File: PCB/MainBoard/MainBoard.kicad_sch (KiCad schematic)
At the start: 15 parts, among them J1 Conn_01x04_12864, J2 Conn_01x03_Female, J3 Conn_01x03_Female, J4 Conn_01x04_12864, J5 Conn_01x04_12864, J6 Conn_02x20_Odd_Even, SW1 RotaryEncoder_Switch, U2 Pico

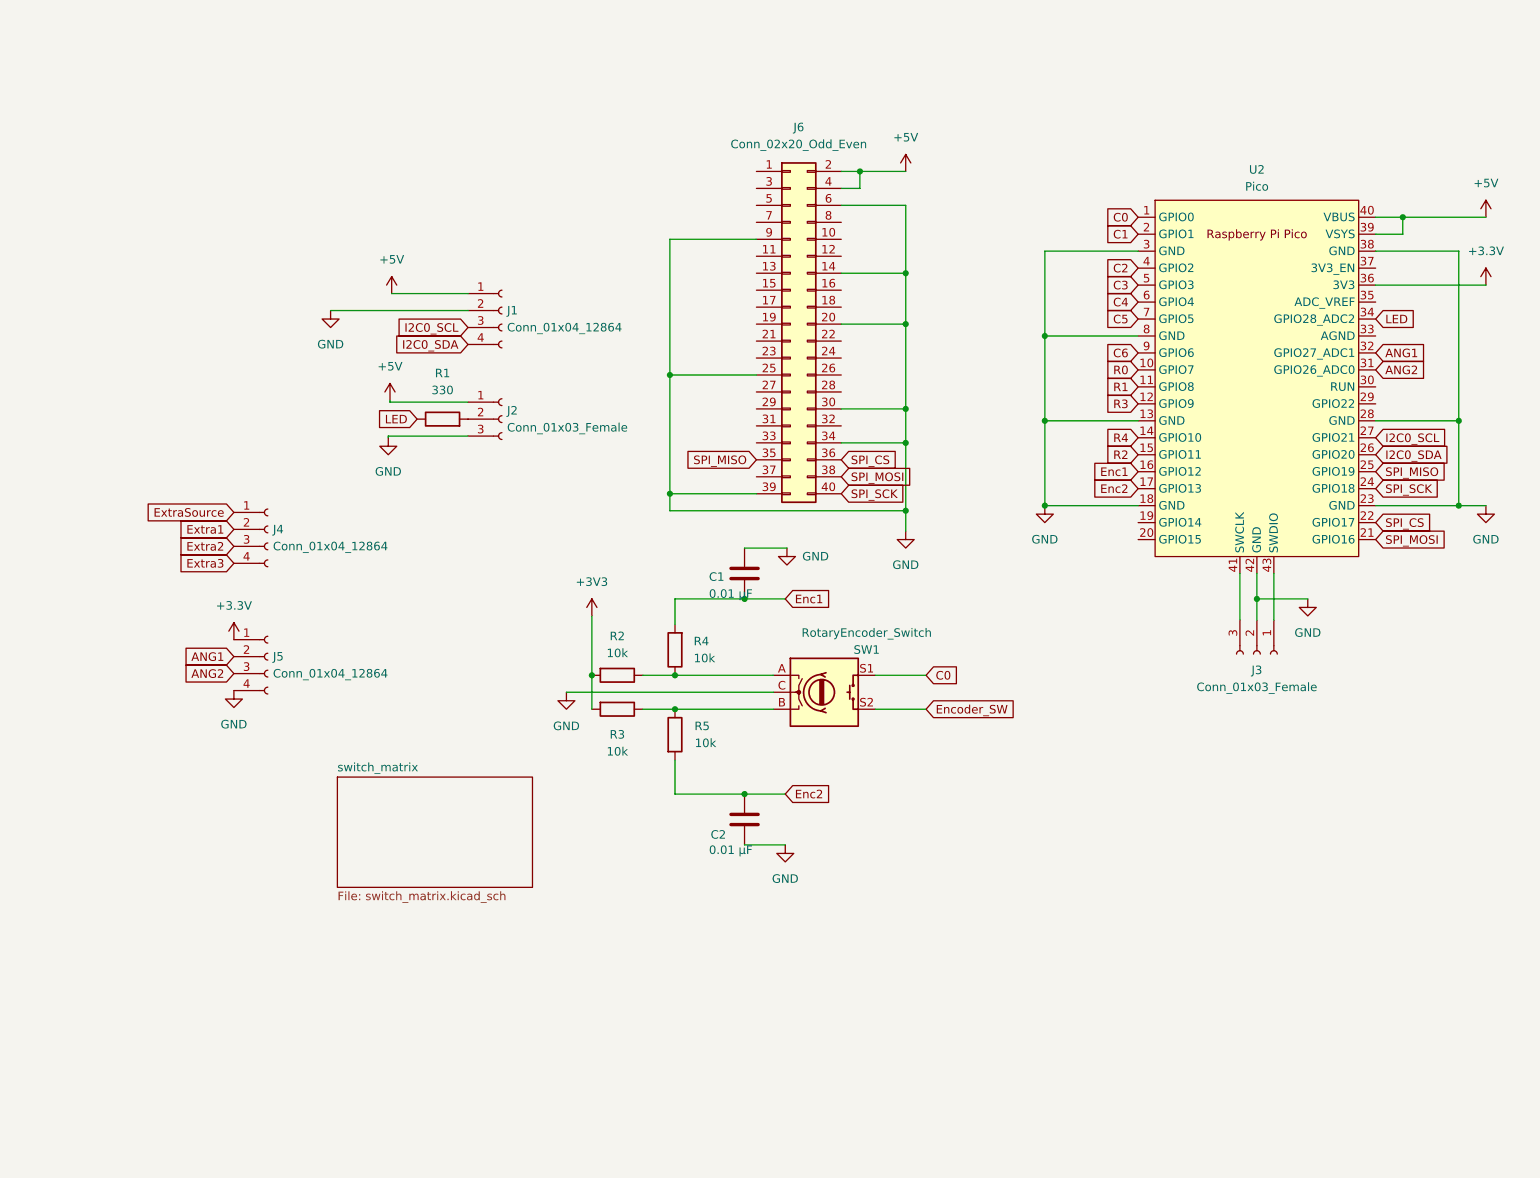
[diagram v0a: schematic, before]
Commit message: Updated 3d model
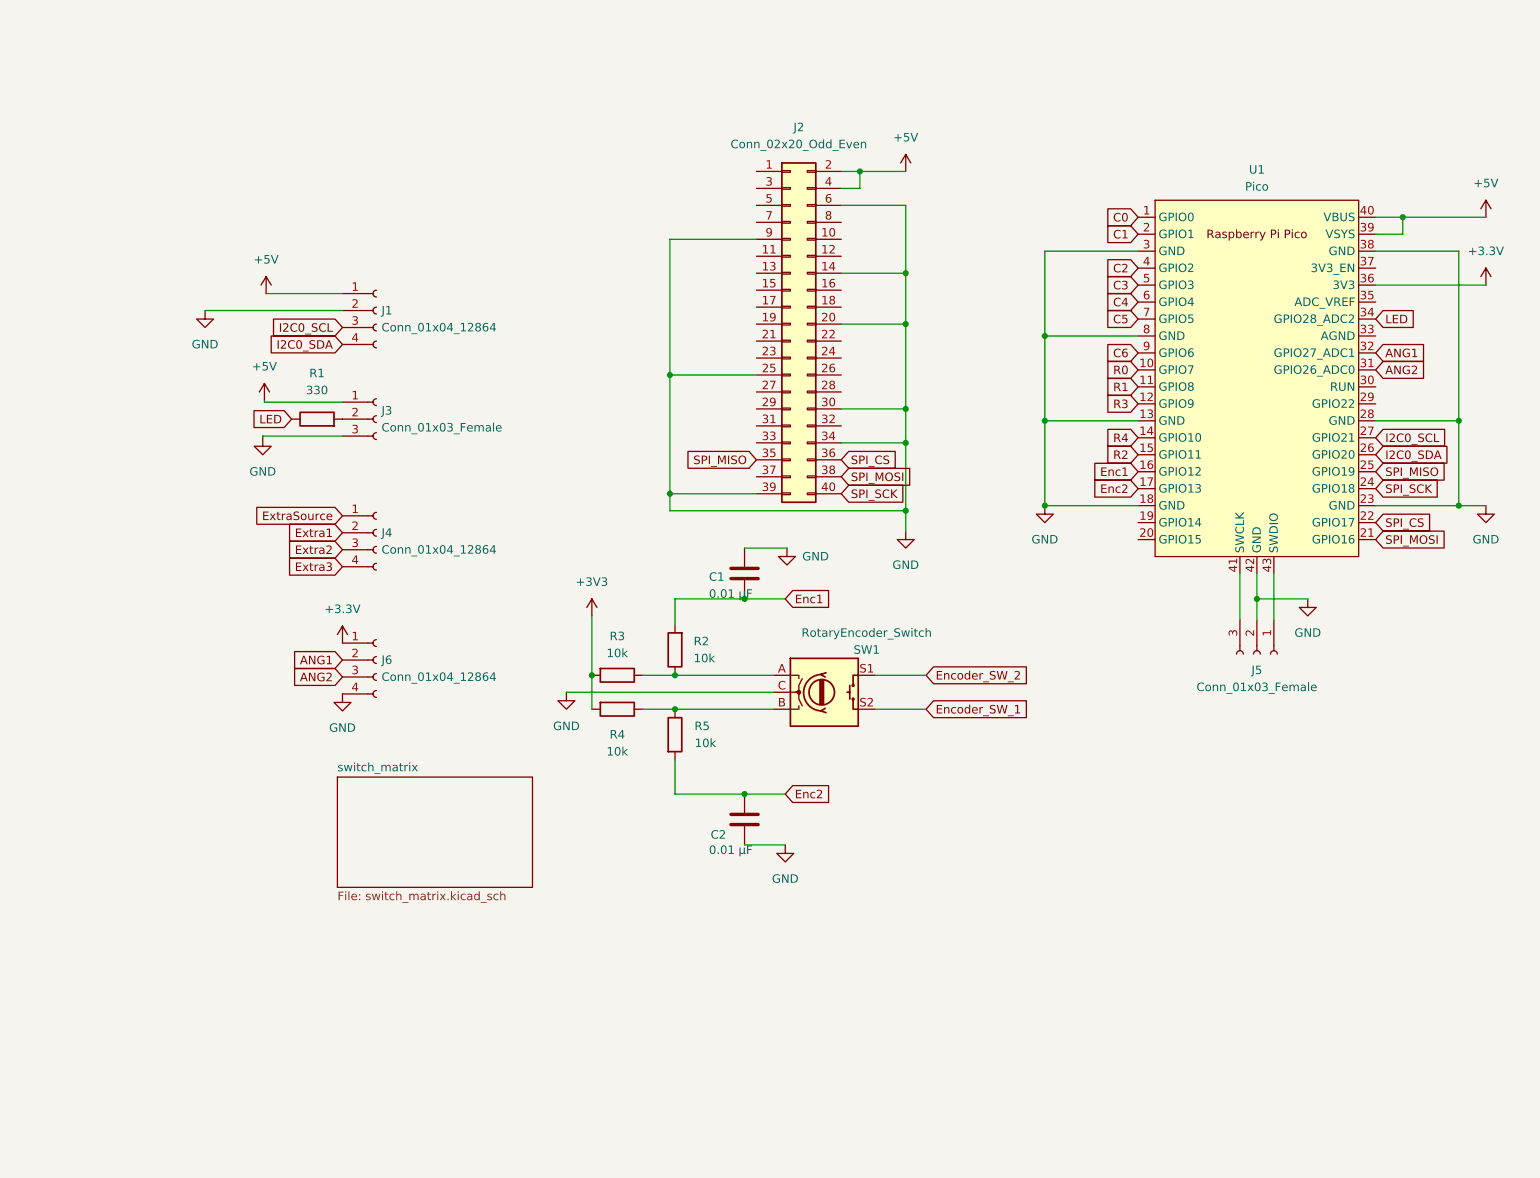
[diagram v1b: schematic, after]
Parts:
- renumbered J6 to J2, J2 to J3, J3 to J5, J5 to J6, R4 to R2, R2 to R3, R3 to R4, U2 to U1
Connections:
- net C0: no longer SW1.S1
- net Encoder_SW renamed Encoder_SW_1
- new net Encoder_SW_2: SW1.S1
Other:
- moved on the sheet: J1, J3, J4, J6, R1

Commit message: Layout settled
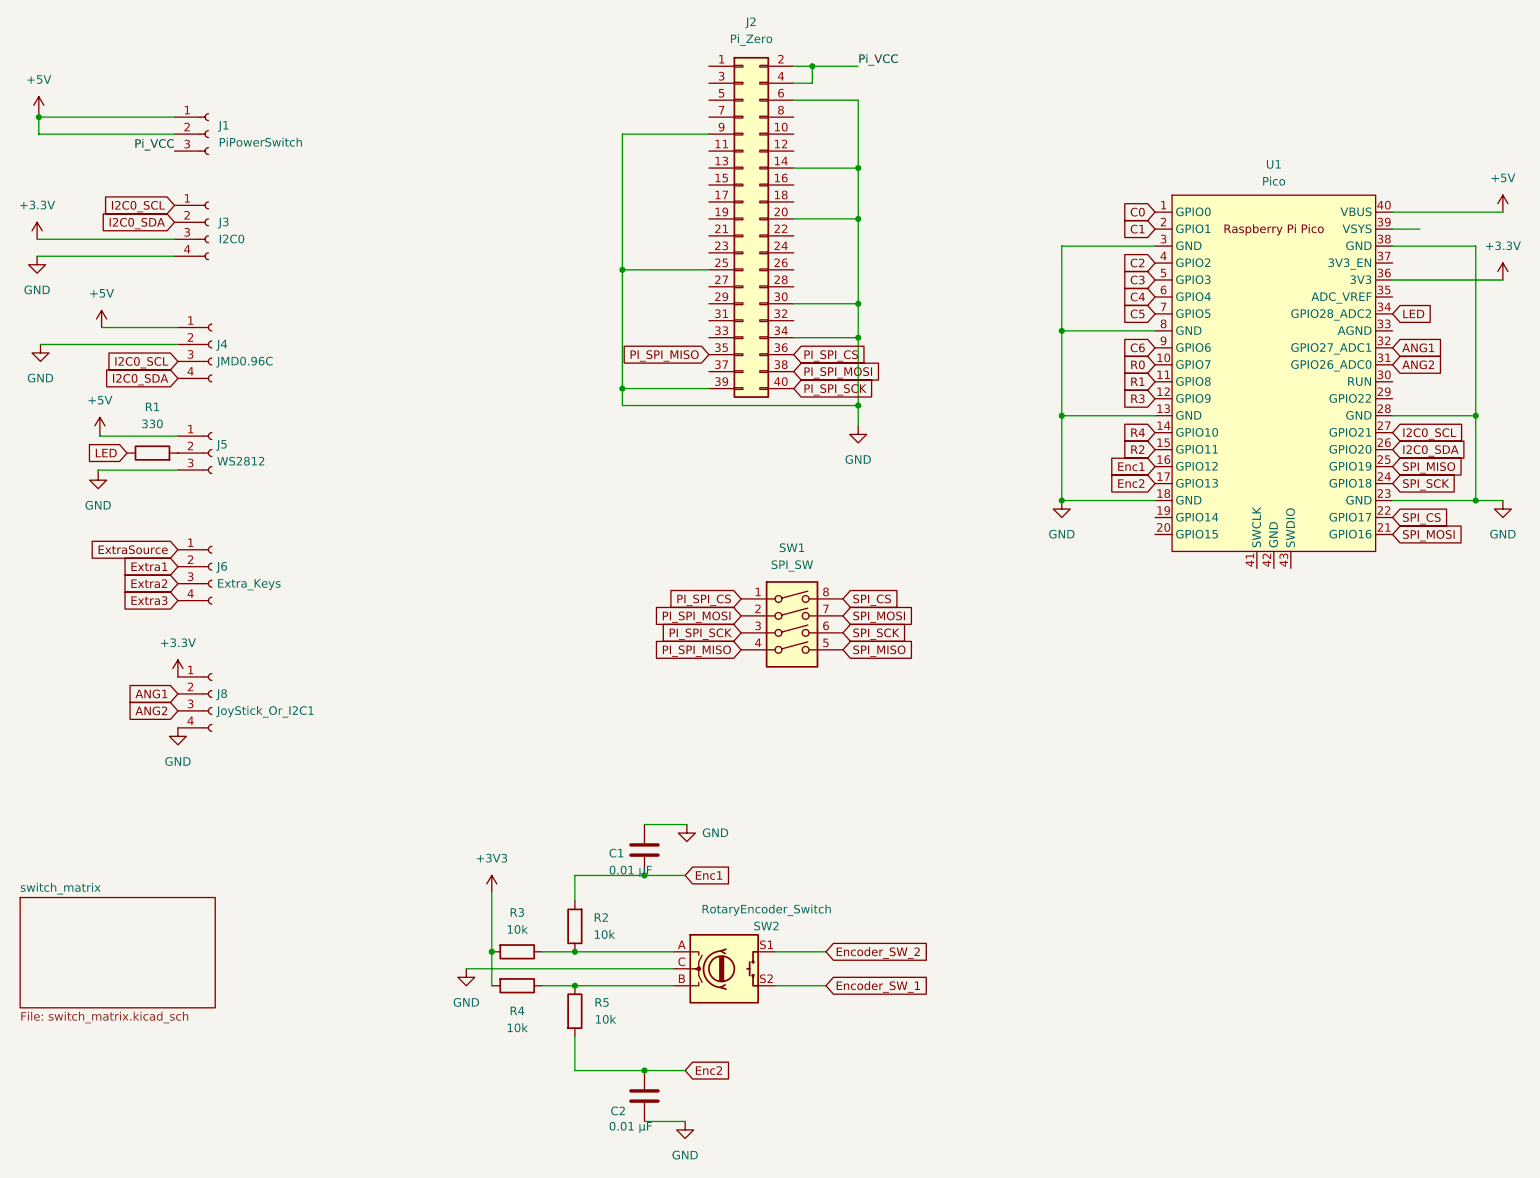
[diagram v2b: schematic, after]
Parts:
- removed J5: Conn_01x03_Female, Connector_PinHeader_2.54mm:PinHeader_1x03_P2.54mm_Vertical, symbol Connector:Conn_01x03_Female
- added J1: PiPowerSwitch, Connector_PinHeader_2.54mm:PinHeader_1x03_P2.54mm_Vertical, symbol Connector:Conn_01x03_Female
- added J3: I2C0, Connector_PinHeader_2.54mm:PinHeader_1x04_P2.54mm_Horizontal, symbol Connector:Conn_01x04_Female
- added SW1: SPI_SW, Button_Switch_THT:SW_DIP_SPSTx04_Slide_6.7x11.72mm_W7.62mm_P2.54mm_LowProfile, symbol Switch:SW_DIP_x04
- J2: value Conn_02x20_Odd_Even -> Pi_Zero
- J4: renamed from J1; value Conn_01x04_12864 -> JMD0.96C
- J5: renamed from J3; value Conn_01x03_Female -> WS2812; footprint Connector_PinHeader_2.54mm:PinHeader_1x03_P2.54mm_Vertical -> Connector_PinHeader_2.54mm:PinHeader_1x03_P2.54mm_Horizontal
- J6: renamed from J4; value Conn_01x04_12864 -> Extra_Keys
- J8: renamed from J6; value Conn_01x04_12864 -> JoyStick_Or_I2C1
- renumbered SW1 to SW2
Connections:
- net +3V3: now also J3.3 (Pin_3)
- net +5V: now also J1.1 (Pin_1), J1.2 (Pin_2); no longer J2.2 (Pin_2), J2.4 (Pin_4), U1.39 (VSYS)
- net GND: now also J3.4 (Pin_4); no longer U1.42 (GND)
- net I2C0_SCL: now also J3.1 (Pin_1)
- net I2C0_SDA: now also J3.2 (Pin_2)
- net SPI_CS: now also SW1.8; no longer J2.36 (Pin_36)
- net SPI_MISO: now also SW1.5; no longer J2.35 (Pin_35)
- net SPI_MOSI: now also SW1.7; no longer J2.38 (Pin_38)
- net SPI_SCK: now also SW1.6; no longer J2.40 (Pin_40)
- new net PI_SPI_CS: J2.36 (Pin_36), SW1.1
- new net PI_SPI_MISO: J2.35 (Pin_35), SW1.4
- new net PI_SPI_MOSI: J2.38 (Pin_38), SW1.2
- new net PI_SPI_SCK: J2.40 (Pin_40), SW1.3
- new net Pi_VCC: J1.3 (Pin_3), J2.2 (Pin_2), J2.4 (Pin_4)
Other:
- moved on the sheet: C1, C2, J2, J4, J5, J6, J8, R1, R2, R3, R4, R5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
